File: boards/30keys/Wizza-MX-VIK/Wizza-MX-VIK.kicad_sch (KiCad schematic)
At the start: 88 parts, among them J1 AudioJack4dpb, J2 AudioJack4dpb, J3 Conn_01x03_Socket, J4 Conn_01x03_Socket, J7 Conn_01x05, J8 Conn_01x05, SW1 SW_Push, SW10 SW_Push, SW11 SW_Push, SW12 SW_Push, SW13 SW_Push, SW14 SW_Push, SW15 SW_Push, SW16 SW_Push, SW17 SW_Push, SW18 SW_Push, SW19 SW_Push, SW2 SW_Push, SW20 SW_Push, SW21 SW_Push, SW22 SW_Push, SW23 SW_Push, SW24 SW_Push, SW25 SW_SPDT, SW26 SW_Push, SW27 SW_Push, SW28 SW_Push, SW29 SW_Push, SW3 SW_Push, SW30 SW_SPDT, SW31 SW_Push, SW32 SW_Push, SW33 SW_Push, SW34 Rotary_Encoder_Switch, SW35 Rotary_Encoder_Switch, SW4 SW_Push, SW40 SW_Push, SW5 SW_Push, SW6 SW_Push, SW7 SW_Push, SW8 SW_Push, SW9 SW_Push, U1 Helios, U2 Helios

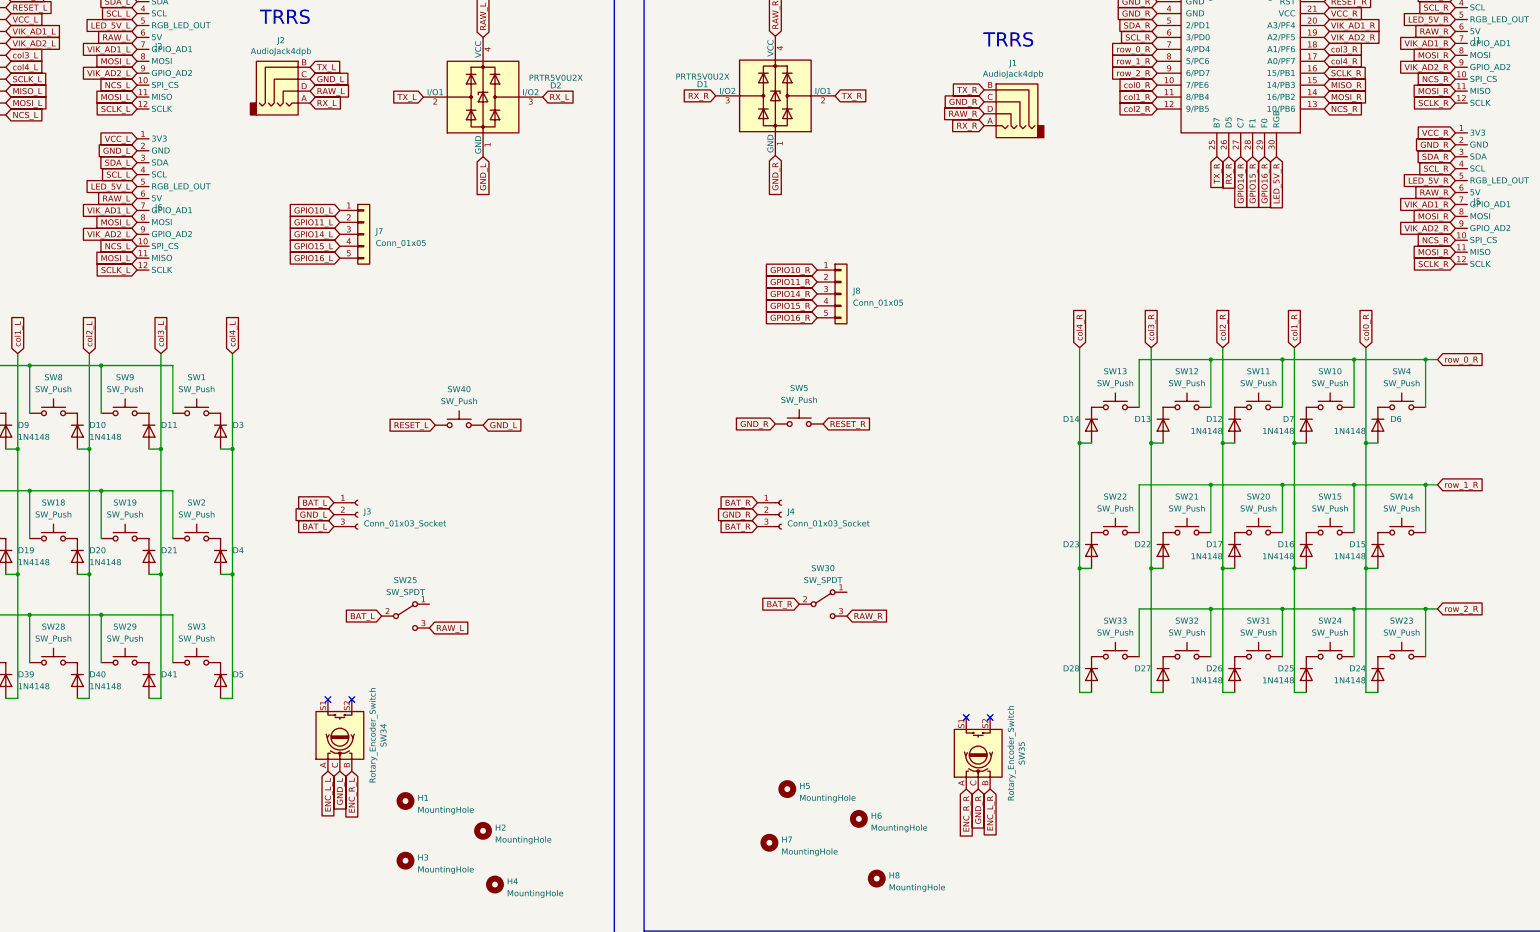
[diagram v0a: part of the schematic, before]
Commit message: wizza mx vik
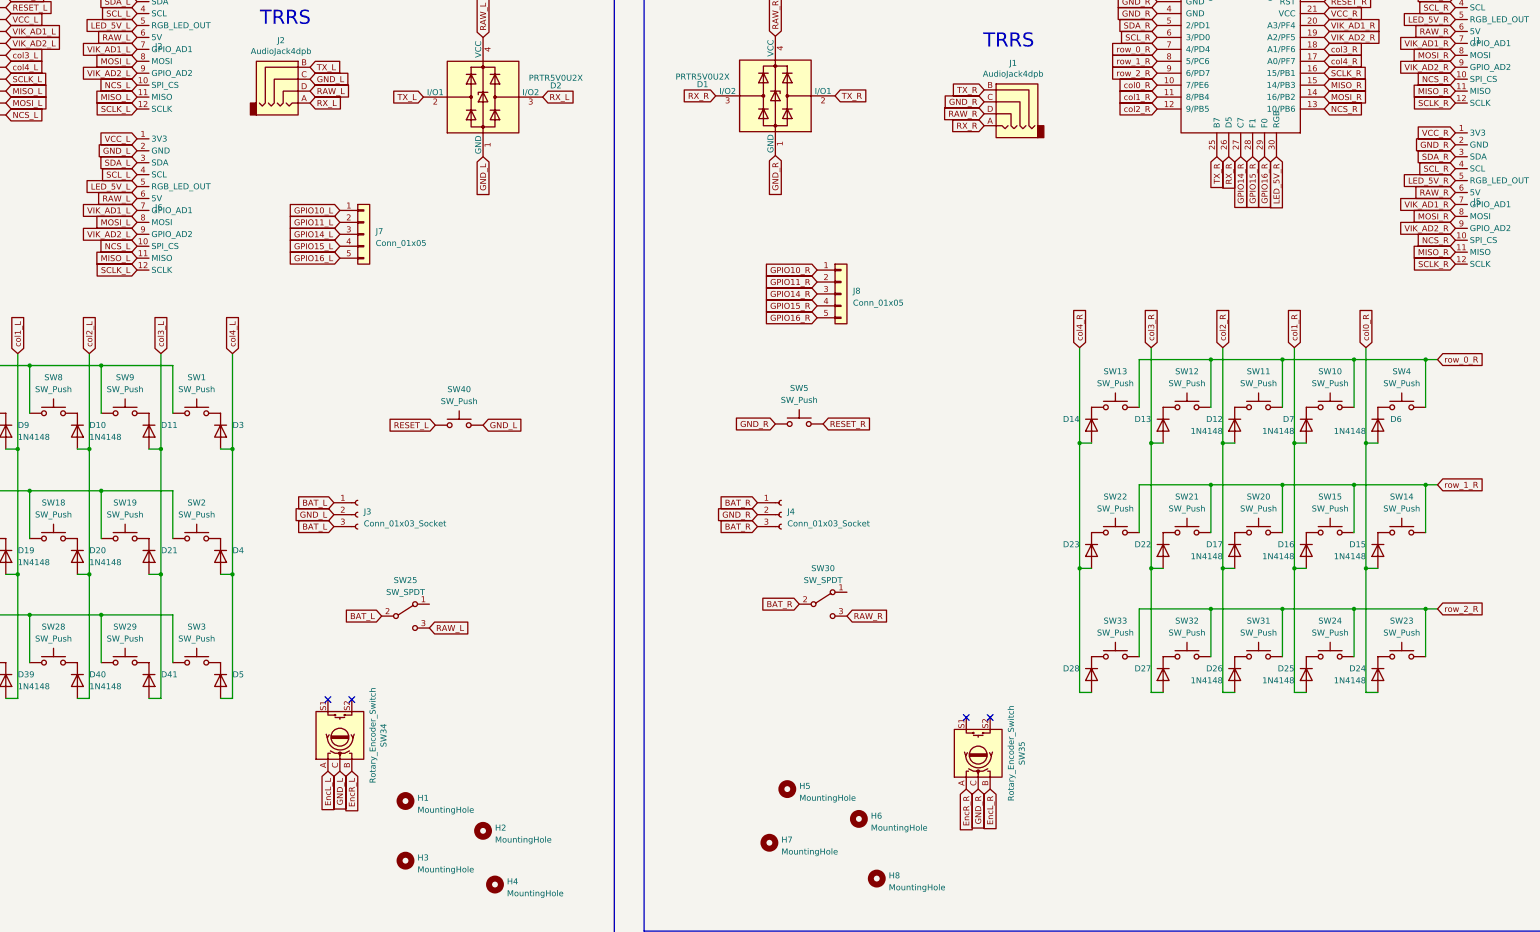
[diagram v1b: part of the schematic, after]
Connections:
- net ENC_L_L is gone; now on net EncL_L: SW34.A
- net ENC_L_R is gone; now on net EncL_R: SW35.B
- net ENC_R_L is gone; now on net EncR_L: SW34.B
- net ENC_R_R is gone; now on net EncR_R: SW35.A
- net MISO_L: now also J2.11 (MISO), J6.11 (MISO)
- net MISO_R: now also J1.11 (MISO), J5.11 (MISO)
- net MOSI_L: no longer J2.11 (MISO), J6.11 (MISO)
- net MOSI_R: no longer J1.11 (MISO), J5.11 (MISO)
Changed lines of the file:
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@@
+    )
+  )
+  (global_label "MISO_R" (shape input) (at 386.08 82.55 180) (fields_autoplaced)
+    (effects (font (size 1.27 1.27)) (justify right))
+    (property "Intersheetrefs" "${INTERSHEET_REFS}" (at 376.3404 82.55 0)
+      (effects (font (size 1.27 1.27)) (justify right) hide)
     )
   )
@@
     )
   )
-  (global_label "MOSI_R" (shape input) (at 386.08 82.55 180) (fields_autoplaced)
-    (effects (font (size 1.27 1.27)) (justify right))
-    (property "Intersheetrefs" "${INTERSHEET_REFS}" (at 376.3404 82.55 0)
-      (effects (font (size 1.27 1.27)) (justify right) hide)
-    )
-  )
   (global_label "NCS_L" (shape input) (at 77.47 87.63 0) (fields_autoplaced)
     (effects (font (size 1.27 1.27)) (justify left))
@@
     )
   )
-  (global_label "MOSI_L" (shape input) (at 105.41 118.11 180) (fields_autoplaced)
-    (effects (font (size 1.27 1.27)) (justify right))
-    (property "Intersheetrefs" "${INTERSHEET_REFS}" (at 95.9123 118.11 0)
-      (effects (font (size 1.27 1.27)) (justify right) hide)
-    )
-  )
   (global_label "GND_L" (shape input) (at 179.07 153.67 0) (fields_autoplaced)
     (effects (font (size 1.27 1.27)) (justify left))
@@
     )
   )
-  (global_label "MOSI_R" (shape input) (at 386.08 116.84 180) (fields_autoplaced)
-    (effects (font (size 1.27 1.27)) (justify right))
-    (property "Intersheetrefs" "${INTERSHEET_REFS}" (at 376.3404 116.84 0)
-      (effects (font (size 1.27 1.27)) (justify right) hide)
-    )
-  )
   (global_label "GND_R" (shape input) (at 322.58 66.04 180) (fields_autoplaced)
     (effects (font (size 1.27 1.27)) (justify right))
@@
     )
   )
-  (global_label "ENC_L_R" (shape input) (at 287.02 231.14 270) (fields_autoplaced)
-    (effects (font (size 1.27 1.27)) (justify right))
-    (property "Intersheetrefs" "${INTERSHEET_REFS}" (at 287.02 242.0286 90)
+  (global_label "EncL_R" (shape input) (at 287.02 231.14 270) (fields_autoplaced)
+    (effects (font (size 1.27 1.27)) (justify right))
+    (property "Intersheetrefs" "${INTERSHEET_REFS}" (at 287.02 240.6981 90)
       (effects (font (size 1.27 1.27)) (justify right) hide)
     )
@@
     )
   )
+  (global_label "MISO_L" (shape input) (at 105.41 118.11 180) (fields_autoplaced)
+    (effects (font (size 1.27 1.27)) (justify right))
+    (property "Intersheetrefs" "${INTERSHEET_REFS}" (at 95.9123 118.11 0)
+      (effects (font (size 1.27 1.27)) (justify right) hide)
+    )
+  )
   (global_label "SCLK_R" (shape input) (at 358.14 78.74 0) (fields_autoplaced)
     (effects (font (size 1.27 1.27)) (justify left))
@@
     )
   )
-  (global_label "ENC_L_L" (shape input) (at 146.05 227.33 270) (fields_autoplaced)
-    (effects (font (size 1.27 1.27)) (justify right))
-    (property "Intersheetrefs" "${INTERSHEET_REFS}" (at 146.05 237.9767 90)
+  (global_label "EncL_L" (shape input) (at 146.05 227.33 270) (fields_autoplaced)
+    (effects (font (size 1.27 1.27)) (justify right))
+    (property "Intersheetrefs" "${INTERSHEET_REFS}" (at 146.05 236.6462 90)
       (effects (font (size 1.27 1.27)) (justify right) hide)
     )
@@
     )
   )
+  (global_label "MISO_R" (shape input) (at 386.08 116.84 180) (fields_autoplaced)
+    (effects (font (size 1.27 1.27)) (justify right))
+    (property "Intersheetrefs" "${INTERSHEET_REFS}" (at 376.3404 116.84 0)
+      (effects (font (size 1.27 1.27)) (justify right) hide)
+    )
+  )
   (global_label "EncL_R" (shape input) (at 322.58 60.96 180) (fields_autoplaced)
     (effects (font (size 1.27 1.27)) (justify right))
@@
     )
   )
-  (global_label "ENC_R_R" (shape input) (at 281.94 231.14 270) (fields_autoplaced)
-    (effects (font (size 1.27 1.27)) (justify right))
-    (property "Intersheetrefs" "${INTERSHEET_REFS}" (at 281.94 242.2705 90)
-      (effects (font (size 1.27 1.27)) (justify right) hide)
-    )
-  )
-  (global_label "ENC_R_L" (shape input) (at 151.13 227.33 270) (fields_autoplaced)
-    (effects (font (size 1.27 1.27)) (justify right))
-    (property "Intersheetrefs" "${INTERSHEET_REFS}" (at 151.13 238.2186 90)
-      (effects (font (size 1.27 1.27)) (justify right) hide)
-    )
-  )
-  (global_label "MOSI_L" (shape input) (at 105.41 83.82 180) (fields_autoplaced)
+  (global_label "EncR_R" (shape input) (at 281.94 231.14 270) (fields_autoplaced)
+    (effects (font (size 1.27 1.27)) (justify right))
+    (property "Intersheetrefs" "${INTERSHEET_REFS}" (at 281.94 240.94 90)
+      (effects (font (size 1.27 1.27)) (justify right) hide)
+    )
+  )
+  (global_label "EncR_L" (shape input) (at 151.13 227.33 270) (fields_autoplaced)
+    (effects (font (size 1.27 1.27)) (justify right))
+    (property "Intersheetrefs" "${INTERSHEET_REFS}" (at 151.13 236.8881 90)
+      (effects (font (size 1.27 1.27)) (justify right) hide)
+    )
+  )
+  (global_label "MISO_L" (shape input) (at 105.41 83.82 180) (fields_autoplaced)
     (effects (font (size 1.27 1.27)) (justify right))
     (property "Intersheetrefs" "${INTERSHEET_REFS}" (at 95.9123 83.82 0)
